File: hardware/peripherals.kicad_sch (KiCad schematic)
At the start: 9 parts, among them J1 Conn_01x02, U1 MAX98357A

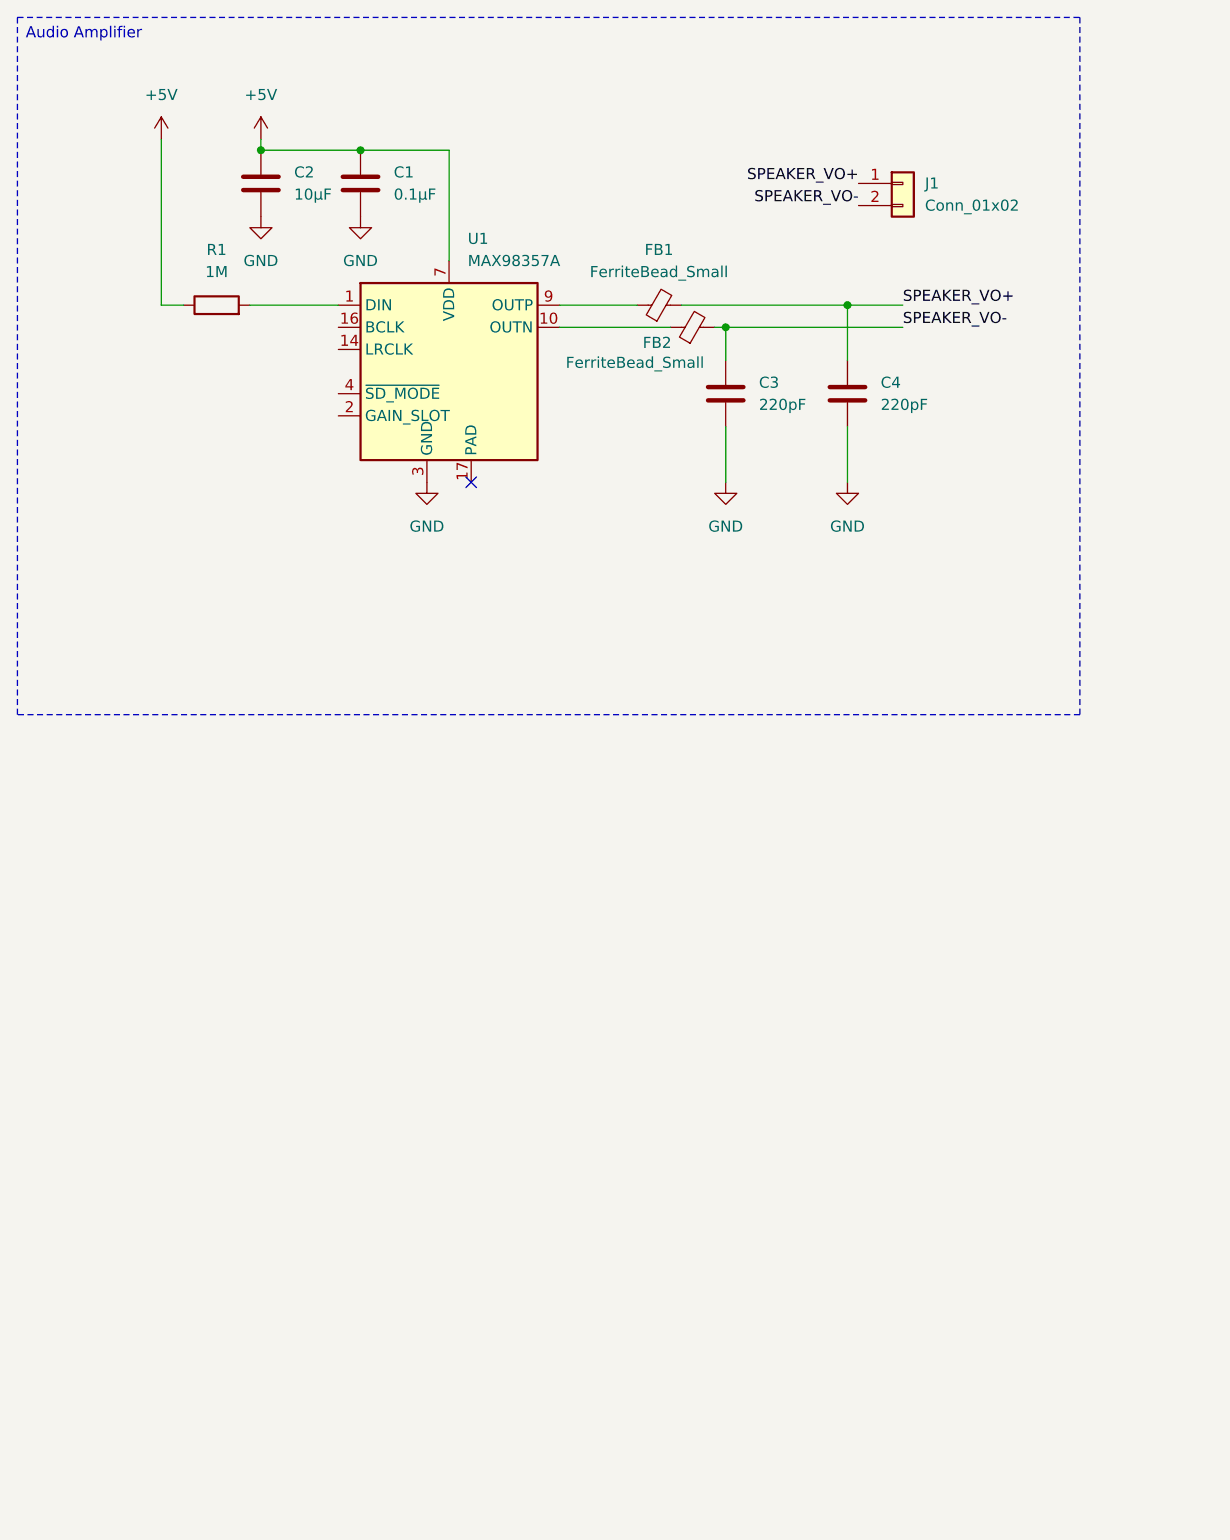
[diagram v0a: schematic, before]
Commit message: Adding IMU
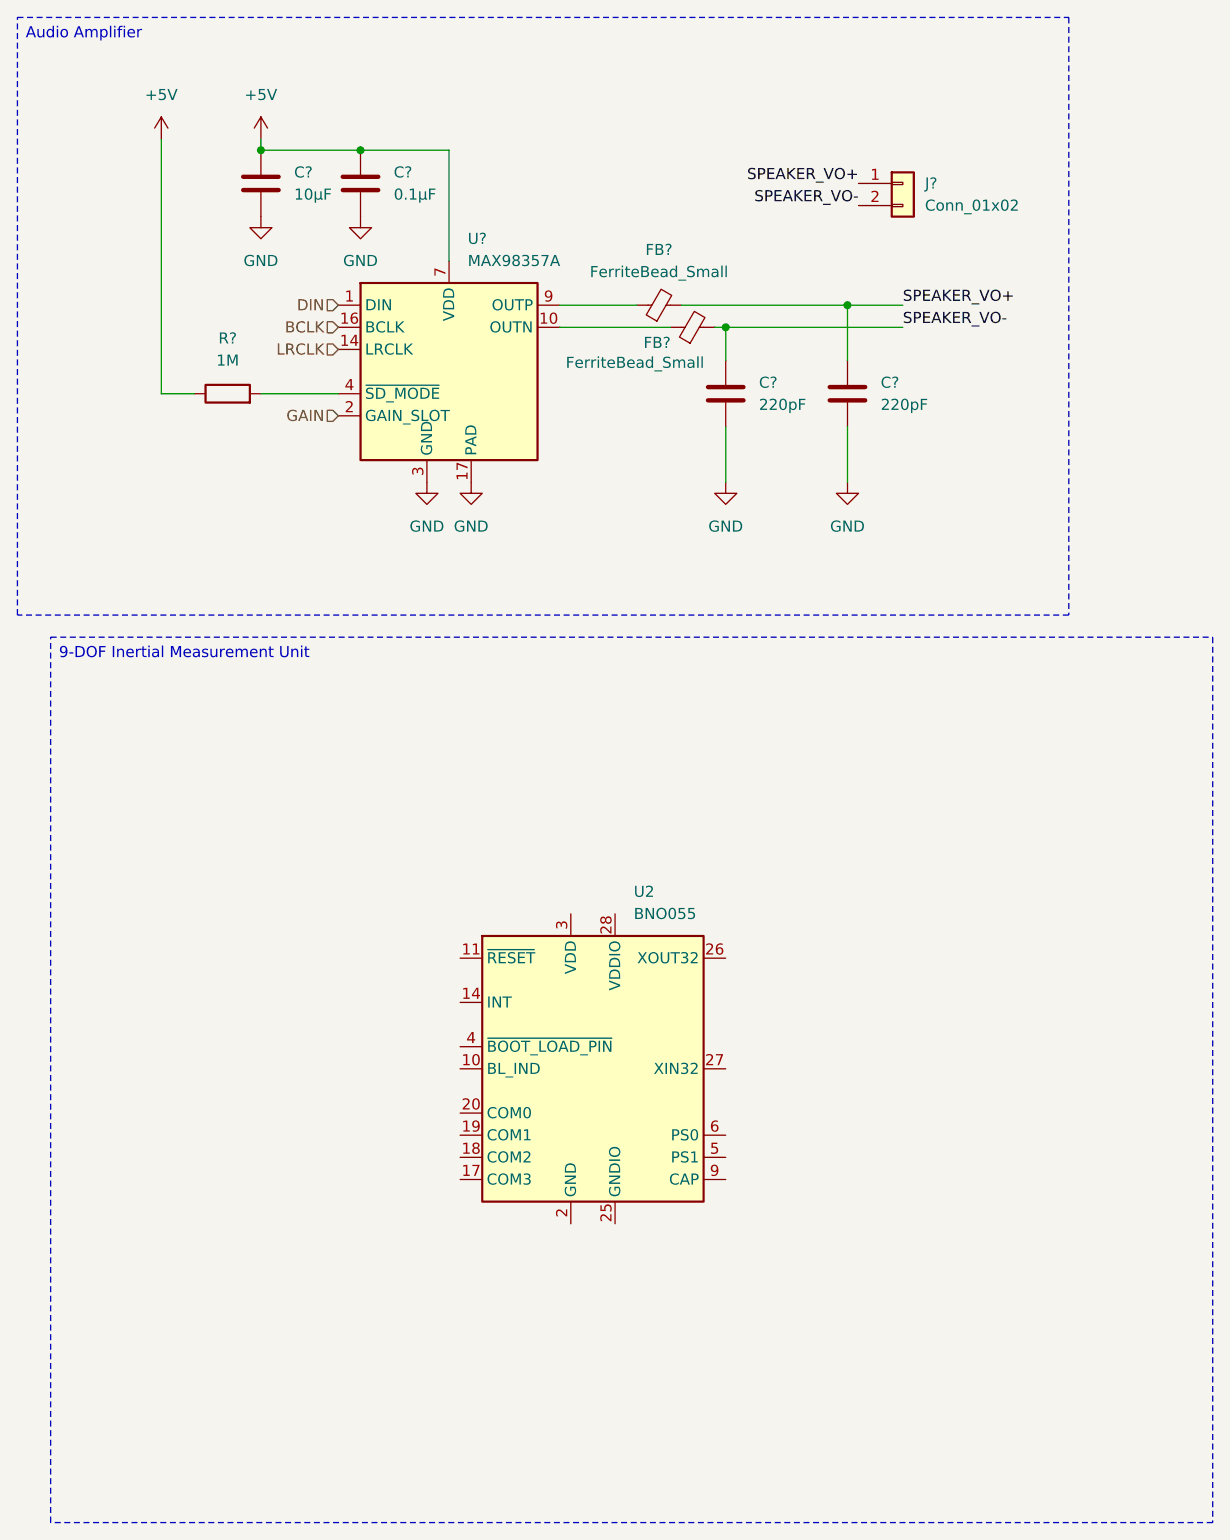
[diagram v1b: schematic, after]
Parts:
- added U2: BNO055, Package_LGA:LGA-28_5.2x3.8mm_P0.5mm, symbol Sensor_Motion:BNO055
- renumbered C4 to C?, C2 to C?, C3 to C?, C1 to C?, FB1 to FB?, FB2 to FB?, J1 to J?, R1 to R?, U1 to U?
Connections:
- net GND: now also U?.17 (PAD)
- net at R?.2: now also U?.4 (~{SD_MODE}); no longer U?.1 (DIN)
- net LRCLK: now reaches U?.14 (LRCLK)
- net BCLK: now reaches U?.16 (BCLK)
- net GAIN: now reaches U?.2 (GAIN_SLOT)
- new net DIN: U?.1 (DIN)
- no-connect marks 1 -> 0
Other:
- moved on the sheet: R?
